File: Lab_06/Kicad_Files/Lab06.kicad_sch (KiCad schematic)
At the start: 5 parts

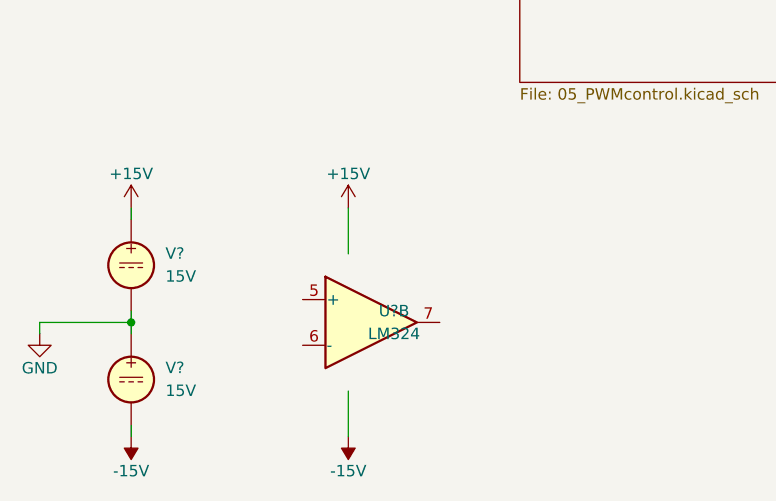
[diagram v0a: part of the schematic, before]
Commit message: Begin Saturday Schematic
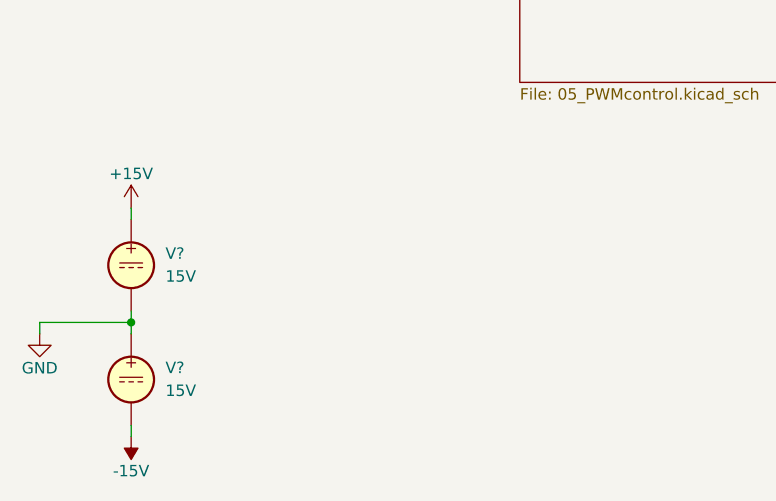
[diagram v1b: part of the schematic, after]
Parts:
- removed U?: LM324, symbol Amplifier_Operational:LM324
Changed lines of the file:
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@@
-    (stroke (width 0) (type default))
-  )
-  (wire (pts (xy 59.69 273.05) (xy 59.69 267.97))
     (stroke (width 0) (type default))
   )
@@
   )
   (wire (pts (xy 200.66 68.58) (xy 217.17 68.58))
-    (stroke (width 0) (type default))
-  )
-  (wire (pts (xy 59.69 252.73) (xy 59.69 247.65))
     (stroke (width 0) (type default))
   )
@@
         (path "/37d0ecfa-1973-4a3c-8fc1-f7066c204731"
           (reference "#PWR04") (unit 1)
-        )
-      )
-    )
-  )
-  (symbol (lib_id "power:+15V") (at 59.69 247.65 0) (unit 1)
-    (in_bom yes) (on_board yes) (dnp no)
-    (property "Reference" "#PWR01" (at 59.69 251.46 0)
-      (effects (font (size 1.27 1.27)) hide)
-    )
-    (property "Value" "+15V" (at 59.69 243.84 0)
-      (effects (font (size 1.27 1.27)))
-    )
-    (property "Footprint" "" (at 59.69 247.65 0)
-      (effects (font (size 1.27 1.27)) hide)
-    )
-    (property "Datasheet" "" (at 59.69 247.65 0)
-      (effects (font (size 1.27 1.27)) hide)
-    )
-    (pin "1")
-    (instances
-      (project "Lab06"
-        (path "/37d0ecfa-1973-4a3c-8fc1-f7066c204731"
-          (reference "#PWR01") (unit 1)
         )
       )
@@
     )
   )
-  (symbol (lib_id "power:-15V") (at 59.69 273.05 0) (mirror x) (unit 1)
-    (in_bom yes) (on_board yes) (dnp no)
-    (property "Reference" "#PWR02" (at 59.69 275.59 0)
-      (effects (font (size 1.27 1.27)) hide)
-    )
-    (property "Value" "-15V" (at 59.69 276.86 0)
-      (effects (font (size 1.27 1.27)))
-    )
-    (property "Footprint" "" (at 59.69 273.05 0)
-      (effects (font (size 1.27 1.27)) hide)
-    )
-    (property "Datasheet" "" (at 59.69 273.05 0)
-      (effects (font (size 1.27 1.27)) hide)
-    )
-    (pin "1")
-    (instances
-      (project "Lab06"
-        (path "/37d0ecfa-1973-4a3c-8fc1-f7066c204731"
-          (reference "#PWR02") (unit 1)
-        )
-      )
-    )
-  )
   (symbol (lib_id "Simulation_SPICE:VDC") (at 35.56 266.7 0) (unit 1)
     (in_bom yes) (on_board yes) (dnp no) (fields_autoplaced)
@@
         )
       )
-    )
-  )
-  (symbol (lib_id "Amplifier_Operational:LM324") (at 62.23 260.35 0) (unit 2)
-    (in_bom yes) (on_board yes) (dnp no)
-    (property "Reference" "U?" (at 64.77 259.08 0)
-      (effects (font (size 1.27 1.27)))
-    )
-    (property "Value" "LM324" (at 64.77 261.62 0)
-      (effects (font (size 1.27 1.27)))
-    )
-    (property "Footprint" "" (at 60.96 257.81 0)
-      (effects (font (size 1.27 1.27)) hide)
-    )
-    (property "Datasheet" "http://www.ti.com/lit/ds/symlink/lm2902-n.pdf" (at 63.5 255.27 0)
-      (effects (font (size 1.27 1.27)) hide)
-    )
-    (pin "1")
-    (pin "2")
-    (pin "3")
-    (pin "5")
-    (pin "6")
-    (pin "7")
-    (pin "10")
-    (pin "8")
-    (pin "9")
-    (pin "12")
-    (pin "13")
-    (pin "14")
-    (pin "11")
-    (pin "4")
-    (instances
-      (project "Lab06"
-        (path "/37d0ecfa-1973-4a3c-8fc1-f7066c204731/38fa6eb6-6b75-4a2f-a07b-650c2dba198f"
-          (reference "U?") (unit 2)
-        )
-        (path "/37d0ecfa-1973-4a3c-8fc1-f7066c204731"
-          (reference "U401") (unit 5)
-        )
-      )

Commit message: Continue Lab 6 Saturday Schematic
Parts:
- added J? (x3): Banana Socket, symbol Connector:Conn_01x01_Socket
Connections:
- net GND: now also J?.1 (Pin_1)
- net Square and Triangle Oscillator/SQUARE_OUT: now reaches SW?.1
- net Pulse Width Control Circuitry/TRIANGLE_IN: now reaches SW?.2
- net Sinewave Shaper/SINE_OUT: now reaches SW?.3
- net PWM: now reaches SW?.10
- net PWM: now also SW?.11, SW?.12
- net at SW?.14: now also J?.1 (Pin_1)
- net Primary Drive Circuitry/Waveform_In renamed Primary Drive Circuitry/WAVEFORM_IN
- net SIN_OUT renamed SIN
- new net Pulse Width Control Circuitry/GATE_IN: J?.1 (Pin_1)
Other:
- sheet Primary Drive Circuitry ports: added WAVEFORM_IN, WAVEFORM_OUT; removed Waveform_In, Waveform_Out
- sheet Pulse Output Drive Circuitry ports: added PULSE_IN, PULSE_OUT; removed none
- sheet Pulse Width Control Circuitry ports: added GATE_IN, PULSE_OUT, TRIANGLE_IN; removed none
- sheet Sinewave Shaper ports: added SINE_OUT, TRIANGLE_IN; removed none
- sheet Square and Triangle Oscillator ports: added GATE_IN, SQUARE_OUT, TRIANGLE_OUT; removed none
- note added: "Gate Input"
- note added: "Output"
- note added: "Waveform Select"
- moved on the sheet: SW?A, SW?B, V?

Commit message: Finish Saturday Schematic
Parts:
- removed V? (x2): 15V, symbol Simulation_SPICE:VDC
- added C1, C2: 0.01uF, symbol Device:C
- added C3, C4: 220uF, symbol Device:C_Polarized_US
- added J2, J3, J4: Banana Socket, symbol Connector:Conn_01x01_Socket
- gave numbers to parts that had none: 4
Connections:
- net Pulse Width Control Circuitry/TRIANGLE_IN is gone; now on net SIN: SW1.2
- net Sinewave Shaper/SINE_OUT is gone; now on net SIN: SW1.3
- net Square and Triangle Oscillator/SQUARE_OUT is gone; now on net SIN: SW1.1
- net +15V: now also C1.1, C3.1, J2.1 (Pin_1)
- net -15V: now also C2.2, C4.2, J4.1 (Pin_1)
- net GND: now also C1.2, C2.1, C3.2, C4.1, J3.1 (Pin_1)
- net Pulse Width Control Circuitry/GATE_IN renamed Square and Triangle Oscillator/GATE_IN
- no-connect marks 0 -> 3
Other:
- sheet Pulse Width Control Circuitry ports: added none; removed GATE_IN
- note added: "BLACK"
- note added: "BLUE"
- note added: "Power Input"
- note added: "RED"
- note added: "YELLOW"
- moved on the sheet: J1

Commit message: Revise Schematic
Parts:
- removed SW1: ~, symbol Lab06:371_SW_Rotary2x6
- added C201: 0.22uF, symbol Device:C
- added C202: 0.022uF, symbol Device:C
- added C601: 1000pF, symbol Device:C
- added D201, D202, D203, D204: ~, symbol Lab06:D_45
- added D301, D302: D, symbol Device:D
- added Q201 (x3): PNP, symbol Simulation_SPICE:PNP
- added Q202 (x3), Q203, Q204, Q601: NPN, symbol Simulation_SPICE:NPN
- added R201 (x3), R203, R205, R207 (x3), R208, R209, R214, R601: 1K, symbol Device:R
- added R202, R210, R215: 10K, symbol Device:R
- added R204, R206: R, symbol Device:R
- added R206 (x2): 4K7, symbol Device:R
- added R211: 3K3, symbol Device:R
- added R211: 27K, symbol Device:R
- added R212: 5K6, symbol Device:R
- added R213: 47K, symbol Device:R
- added R301, R602: 220R, symbol Device:R
- added R4: 68K, symbol Device:R
- added R4: 33K, symbol Device:R
- added R501: 2K2, symbol Device:R
- added RV201: 1K, symbol Device:R_Potentiometer_Trim
- added RV201: 100K, symbol Device:R_Potentiometer
- added RV201 (x3): 10K, symbol Device:R_Potentiometer
- added RV201: 1K, symbol Device:R_Potentiometer
- added RV202: 10K, symbol Device:R_Potentiometer_Trim
- added SW2: ~, symbol Lab06:371_SW_Rotary2x6
- added SW201: RANGE, symbol Lab06:SW_SPDT
- added U201, U401: LM324A, symbol Amplifier_Operational:LM324A
- added U501: LM393, symbol Comparator:LM393
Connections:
- net +15V: now also Q201.3 (E), Q201.3 (E), R207.1, R207.1, R501.1, R602.1, RV201.1, RV201.1, RV202.1, U201.4 (V+), U401.4 (V+), U501.8 (V+)
- net -15V: now also Q202.3 (E), Q202.3 (E), R207.1, R208.2, RV202.3, U201.11 (V-), U401.11 (V-)
- net GND: now also C201.2, C202.2, D301.1 (K), D302.2 (A), Q203.3 (E), Q204.3 (E), Q601.3 (E), R204.2, R210.2, R211.2, R211.2, R215.2, R4.2, RV201.3, RV201.3, RV201.3, RV201.3, RV201.3, U201.12 (+), U401.5 (+), U501.4 (V-)
- net PWM: now also SW2.10, SW2.11, SW2.12
- net SIN: now also Q201.1 (C), Q202.1 (C), Q204.1 (C), R211.1, R213.2, R301.1, SW2.1, SW2.2, SW2.3, SW2.7, SW2.8, SW2.9, U201.1, U201.2 (-), U201.6 (-), U401.13 (-), U501.2 (-)
- net at J5.1 (Pin_1): now also SW2.14
- net Square and Triangle Oscillator/GATE_IN: no longer names the net of J1.1 (Pin_1)
- net Square and Triangle Oscillator/GATE_IN: now also R209.1, R214.1
- new net: Q203.2 (B), R209.2, R210.1
- new net: D301.2 (A), D302.1 (K), R301.2
- new net: Q201.2 (B), Q202.2 (B), Q601.1 (C), RV201.2
- new net: C601.2, Q601.2 (B), R601.2
- new net: D201.1 (K), D202.2 (A), R212.2, R213.1, U201.7
- new net: Q201.2 (B), Q202.2 (B), U401.14
- new net: SW2.13, U401.3 (+)
- new net: R202.2, R203.2, R205.1, U201.13 (-)
- new net: R205.2, R206.1, U201.14
- new net: C201.1, SW201.1 (A)
- new net: R211.1, R212.1, U201.5 (+)
- new net: Q204.2 (B), R214.2, R215.1
- new net: D203.1 (K), D204.2 (A), Q203.1 (C), SW201.2 (B), U201.3 (+)
- new net: D202.1 (K), D204.1 (K), Q202.1 (C)
- new net: Q202.2 (B), R206.2, R207.2
- new net: Q202.3 (E), R208.1
- new net: R202.1, RV202.2
- new net: R4.2, RV201.1
- new net: RV201.2, U401.2 (-)
- new net: R4.1, RV201.3
- new net: R201.1, R201.2, R201.2, U401.6 (-)
- new net: R201.2, U401.12 (+), U401.7
- new net: R204.1, R206.1
- new net: R4.1, RV201.1, U401.1
- new net: Q201.3 (E), R207.2
- new net: RV201.2, U501.3 (+)
- new net: R203.1, RV201.2, U201.10 (+)
- new net: RV201.2, U401.10 (+)
- new net: C202.1, SW201.3 (C)
- new net: D201.2 (A), D203.2 (A), Q201.1 (C)
- new net: R201.1, RV201.2
- new net: R201.1, U401.8, U401.9 (-)
- new net: R602.2, RV201.1
- new net: Q201.2 (B), R206.2, R207.2
- new net: R206.1, U201.8, U201.9 (-)
- new net PULSE_IN: C601.1, R601.1
- new net PULSE_OUT: Q201.1 (C), Q202.1 (C), R501.2, RV201.1, U501.1
- new net SINE_OUT: R206.2
- no-connect marks 3 -> 6
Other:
- removed sheet Primary Drive Circuitry
- removed sheet Pulse Output Drive Circuitry
- removed sheet Pulse Width Control Circuitry
- removed sheet Sinewave Shaper
- removed sheet Square and Triangle Oscillator
- note added: "0V to 13.5V"
- note added: "1.4Vpk-pk"
- note added: "10Vpk-pk"
- note added: "2Vpk-pk"
- note added: "Amplitude Adjust"
- note added: "Frequency Adjust"
- note added: "Max ampl. Trim"
- note added: "Offset Adjust"
- note added: "Primary Output Driver"
- note added: "Pulse Width Adjust"
- note added: "Range"
- note added: "Sinewave Converter"
- note added: "Symmetry Trim"
- note added: "Triangle/Square Oscillator"
- moved on the sheet: C1, C2, C3, C4, J1, J2, J3, J4
